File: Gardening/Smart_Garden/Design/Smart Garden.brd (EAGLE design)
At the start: 100 x 80 mm, 68 parts, among them IC1 7809DT, IC2 LM1117-3.3, IC3 7805DT, J1 AUDIO_JACK_TRRSSMD_RA, J2 AUDIO_JACK_TRRSSMD_RA, J3 AUDIO_JACK_TRRSSMD_RA, J4 AUDIO_JACK_TRRSSMD_RA, T1 BC847, T2 BC847, T3 BC847, T4 BC847, U1 ESP-32S, U4 MB6S, X1 22-23-2021, X2 22-23-2021, X3 22-23-2021, X4 22-23-2021, X5 22-23-2021

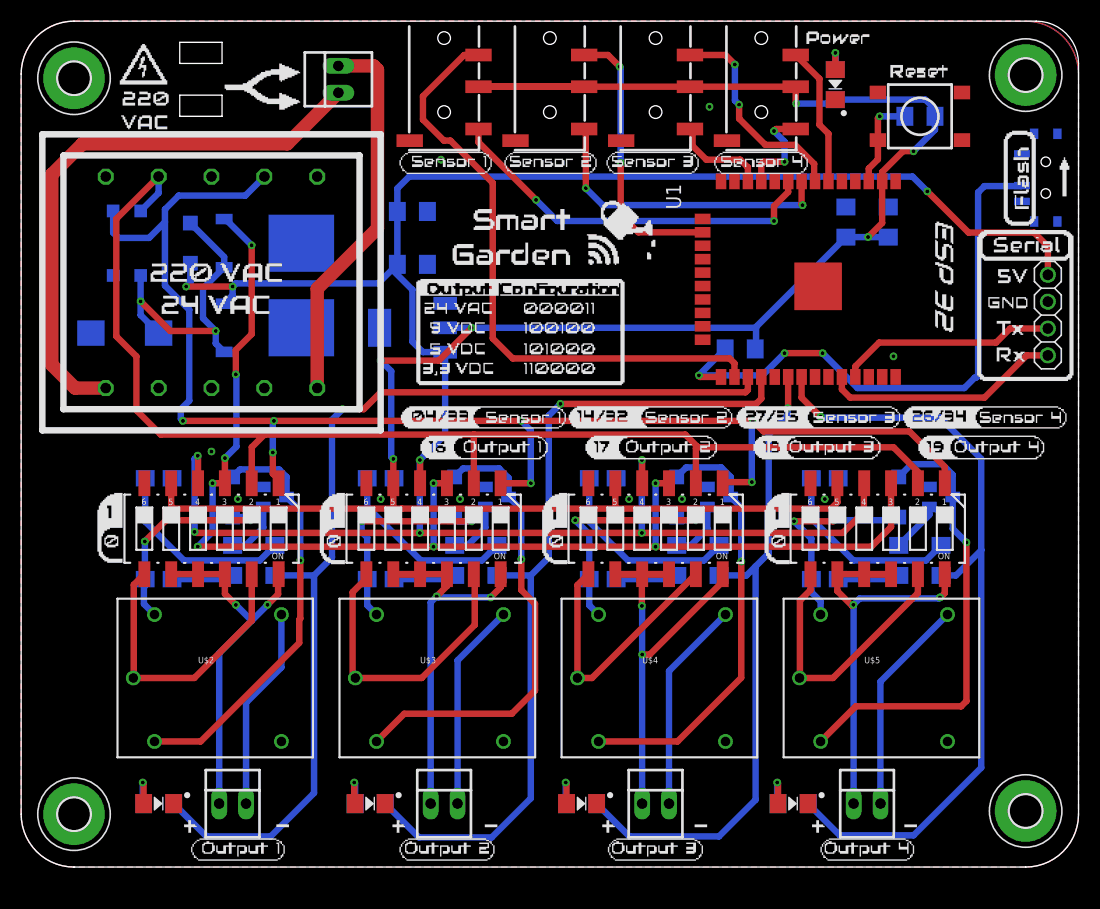
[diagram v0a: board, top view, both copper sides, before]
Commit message: Updated Smart Garden Project docomentation
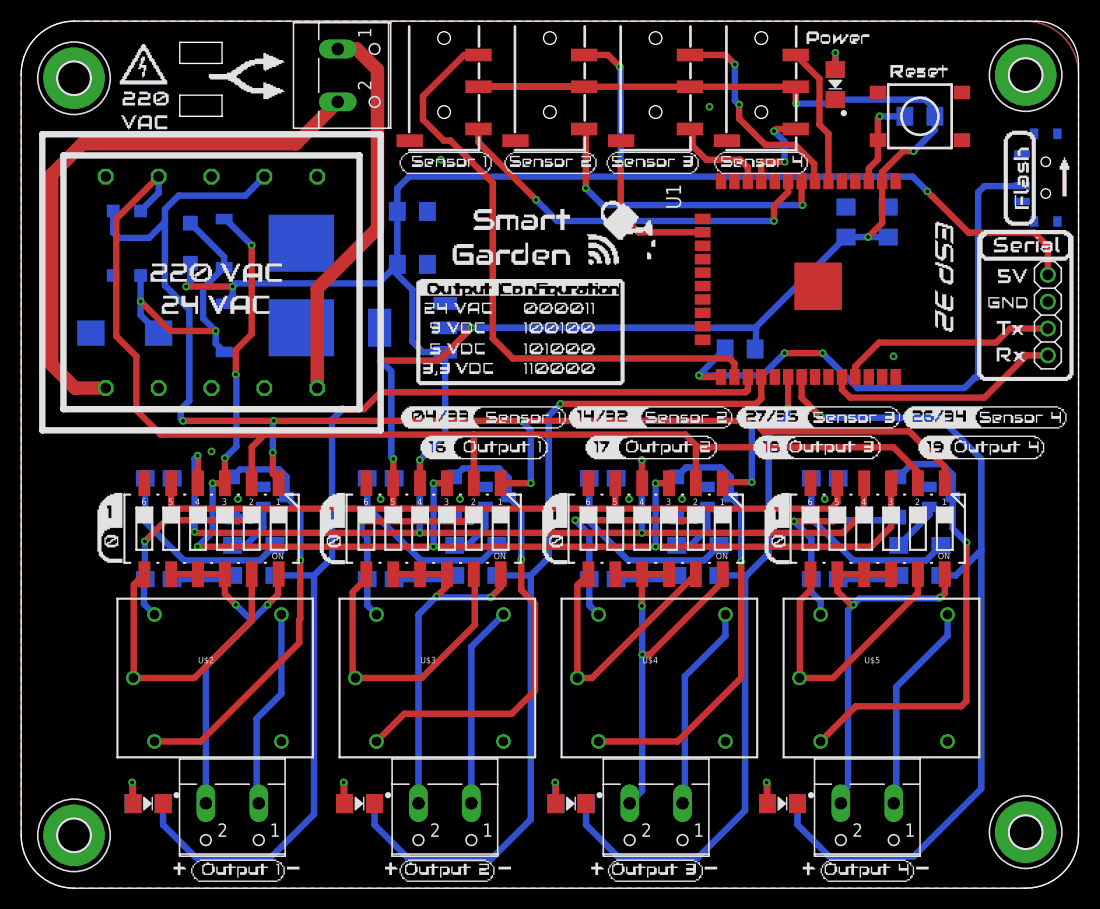
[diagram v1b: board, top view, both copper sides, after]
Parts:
- removed X1, X2, X3, X4, X5: 22-23-2021, con-molex:22-23-2021
- added X10, X6, X7, X8, X9: (no value), con-wago-500:W237-102
- moved H1 2.00 mm to (5.00, 3.00)
- moved H2 2.00 mm to (95.0, 3.30)
- moved L2 1.00 mm to (12.0, 6.00)
- moved L3 1.00 mm to (32.0, 6.00)
- moved L4 1.00 mm to (52.0, 6.00)
- moved L5 1.00 mm to (72.0, 6.00)
- moved R12 1.00 mm to (12.0, 6.00)
- moved R13 1.00 mm to (32.0, 6.00)
- moved R14 1.00 mm to (52.0, 6.00)
- moved R15 1.00 mm to (72.0, 6.00)
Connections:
- net 1R1: now also X7.2; no longer X1.1
- net 2R1: now also X8.2; no longer X2.1
- net 3R1: now also X9.2; no longer X3.1
- net 4R1: now also X10.2; no longer X4.1
- net AC1: now also X6.1; no longer X5.2
- net AC2: now also X6.2; no longer X5.1
- net N$1: now also X10.1; no longer X4.2
- net N$2: now also X9.1; no longer X3.2
- net N$4: now also X8.1; no longer X2.2
- net N$5: now also X7.1; no longer X1.2
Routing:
- net IO19: track 75.7 -> 80.7 mm
- net IO17: track 79.6 -> 84.6 mm
- net IO16: track 97.7 -> 102.7 mm
- net IO18: track 62.8 -> 65.4 mm
- net AC1: track 36.3 -> 37.0 mm
- net N$4: track 19.7 -> 19.1 mm
- net N$2: track 20.1 -> 19.5 mm
- net N$1: track 20.5 -> 20.0 mm
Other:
- board size 100 x 80 mm -> 100 x 82 mm
